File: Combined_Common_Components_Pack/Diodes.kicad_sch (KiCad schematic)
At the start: 8 parts

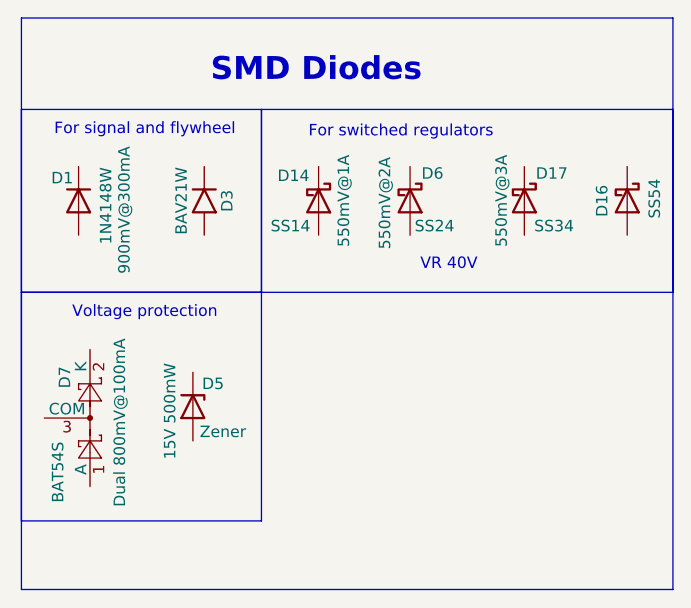
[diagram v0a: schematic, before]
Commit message: More circuits
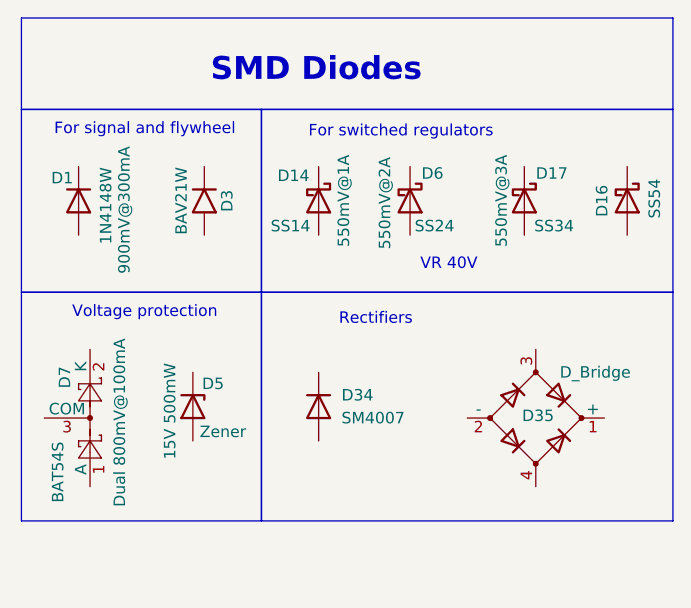
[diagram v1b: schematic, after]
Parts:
- added D34: SM4007, Diode_SMD:D_MELF, symbol Diode:SM4007
- added D35: D_Bridge, Diode_SMD:Diode_Bridge_Diotec_ABS, symbol Device:D_Bridge_+-AA
- D3: Type SMD -> (none)
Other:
- note added: "Rectifiers"
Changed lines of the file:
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@@
 	(rectangle
 		(start 31.75 29.21)
-		(end 104.14 92.71)
+		(end 104.14 39.37)
 		(stroke
 			(width 0)
@@
 		)
 	)
+	(rectangle
+		(start 58.42 59.69)
+		(end 104.14 85.09)
+		(stroke
+			(width 0)
+			(type default)
+		)
+		(fill
+			(type none)
+		)
+	)
 	(text "For switched regulators"
 		(exclude_from_sim no)
 		(at 73.914 41.91 0)
+		(effects
+			(font
+				(size 1.27 1.27)
+			)
+		)
+	)
+	(text "Rectifiers"
+		(exclude_from_sim no)
+		(at 71.12 62.738 0)
 		(effects
 			(font
@@
 	)
 	(symbol
+		(lib_id "Diode:SM4007")
+		(at 64.77 72.39 270)
+		(unit 1)
+		(exclude_from_sim no)
+		(in_bom yes)
+		(on_board yes)
+		(dnp no)
+		(fields_autoplaced yes)
+		(property "Reference" "D34"
+			(at 67.31 71.1199 90)
+			(effects
+				(font
+					(size 1.27 1.27)
+				)
+				(justify left)
+			)
+		)
+		(property "Value" "SM4007"
+			(at 67.31 73.6599 90)
+			(effects
+				(font
+					(size 1.27 1.27)
+				)
+				(justify left)
+			)
+		)
+		(property "Footprint" "Diode_SMD:D_MELF"
+			(at 60.325 72.39 0)
+			(effects
+				(font
+					(size 1.27 1.27)
+				)
+				(hide yes)
+			)
+		)
+		(property "Datasheet" "http://cdn-reichelt.de/documents/datenblatt/A400/SMD1N400%23DIO.pdf"
+			(at 64.77 72.39 0)
+			(effects
+				(font
+					(size 1.27 1.27)
+				)
+				(hide yes)
+			)
+		)
+		(property "Description" "1000V 1A General Purpose Rectifier Diode, MELF"
+			(at 64.77 72.39 0)
+			(effects
+				(font
+					(size 1.27 1.27)
+				)
+				(hide yes)
+			)
+		)
+		(property "Sim.Device" "D"
+			(at 64.77 72.39 0)
+			(effects
+				(font
+					(size 1.27 1.27)
+				)
+				(hide yes)
+			)
+		)
+		(property "Sim.Pins" "1=K 2=A"
+			(at 64.77 72.39 0)
+			(effects
+				(font
+					(size 1.27 1.27)
+				)
+				(hide yes)
+			)
+		)
+		(pin "2"
+		)
+		(pin "1"
+		)
+		(instances
+			(project "Combined_Common_Components_Pack"
+				(path "/59e42e8e-5444-465a-b7a8-ffbd342a8d49/1381f410-15ba-480c-b8e7-d9f156eccb54"
+					(reference "D34")
+					(unit 1)
+				)
+			)
+		)
+	)
+	(symbol
 		(lib_id "Device:D_Zener")
 		(at 50.8 72.39 270)
@@
 			)
 		)
-		(property "Type" "SMD"
-			(at 52.07 49.53 0)
-			(effects
-				(font
-					(size 1.27 1.27)
-				)
-				(hide yes)
-			)
-		)
 		(property "Manufacturer " "MDD(Microdiode Semiconductor)"
 			(at 52.07 49.53 0)
@@
 			)
 		)
-		(property "Sim.Library" ""
-			(at 99.06 49.53 0)
-			(effects
-				(font
-					(size 1.27 1.27)
-				)
-				(hide yes)
-			)
-		)
-		(property "Sim.Name" ""
-			(at 99.06 49.53 0)
-			(effects
-				(font
-					(size 1.27 1.27)
-				)
-				(hide yes)
-			)
-		)
-		(property "Sim.Params" ""
-			(at 99.06 49.53 0)
-			(effects
-				(font
-					(size 1.27 1.27)
-				)
-				(hide yes)
-			)
-		)
 		(property "Manufacturer " "TWGMC"
 			(at 99.06 49.53 0)
@@
 	)
 	(symbol
+		(lib_id "Device:D_Bridge_+-AA")
+		(at 88.9 73.66 0)
+		(unit 1)
+		(exclude_from_sim no)
+		(in_bom yes)
+		(on_board yes)
+		(dnp no)
+		(property "Reference" "D35"
+			(at 89.154 73.406 0)
+			(effects
+				(font
+					(size 1.27 1.27)
+				)
+			)
+		)
+		(property "Value" "D_Bridge"
+			(at 95.504 68.58 0)
+			(effects
+				(font
+					(size 1.27 1.27)
+				)
+			)
+		)
+		(property "Footprint" "Diode_SMD:Diode_Bridge_Diotec_ABS"
+			(at 88.9 73.66 0)
+			(effects
+				(font
+					(size 1.27 1.27)
+				)
+				(hide yes)
+			)
+		)
+		(property "Datasheet" "https://www.lcsc.com/datasheet/C193012.pdf"
+			(at 88.9 73.66 0)
+			(effects
+				(font
+					(size 1.27 1.27)
+				)
+				(hide yes)
+			)
+		)
+		(property "Description" "Diode bridge, +ve/-ve/AC/AC"
+			(at 88.9 73.66 0)
+			(effects
+				(font
+					(size 1.27 1.27)
+				)
+				(hide yes)
+			)
+		)
+		(property "LCSC" "C193012"
+			(at 88.9 73.66 0)
+			(effects
+				(font
+					(size 1.27 1.27)
+				)
+				(hide yes)
+			)
+		)
+		(pin "4"
+		)
+		(pin "1"
+		)
+		(pin "2"
+		)
+		(pin "3"
+		)
+		(instances
+			(project ""
+				(path "/59e42e8e-5444-465a-b7a8-ffbd342a8d49/1381f410-15ba-480c-b8e7-d9f156eccb54"
+					(reference "D35")
+					(unit 1)
+				)
+			)
+		)
+	)
+	(symbol
 		(lib_id "Diode:BAT54S")
 		(at 39.37 73.66 270)
@@
 			(at 38.1 49.53 0)
 			(effects
-				(font
-					(size 1.27 1.27)
-				)
-				(hide yes)
-			)
-		)
-		(property "TYPE" ""
-			(at 38.1 49.53 0)
-			(effects
